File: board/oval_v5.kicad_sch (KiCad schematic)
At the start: 125 parts, among them J1 HDR-5x1, J10 HDR-4x1, J11 HDR-4x1, J12 HDR-4x1, J13 HDR-4x1, J14 HDR-4x1, J15 HDR-4x1, J16 HDR-4x1, J17 HDR-4x1, J18 Conn_Coaxial, J19 Conn_01x02, J2 HDR-4x1, J20 Conn_01x02, J21 Conn_02x02_Counter_Clockwise, J22 HDR-2x1, J23 HDR-2x1, J25 Conn_01x06, J3 HDR-4x1, J4 Conn_01x06, J5 Micro_SD_Card, J6 Conn_01x02, J7 HDR-4x1, J8 Conn_01x08, J9 HDR-4x1, P1 USB_C_Plug_USB2.0, Q1 Q_PMOS_GSD, Q2 MMBT3904, Q3 MMBT3904, SW1 SW_DIP_x02, SW2 SW_DIP_x02, U1 RV-8803, U10 SiP32431DR3, U11 SiP32431DR3, U12 SiP32431DR3, U13 SiP32431DR3, U14 SiP32431DR3, U15 PCF8574TS, U16 PCA9548APW, U17 SiP32431DR3, U2 ESP32-S3-WROOM-1, U3 TMP117xxDRV, U4 RFM95W-915S2, U7 MAX3485, U8 AP7361C-33E, U9 AP7361C-33E

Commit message: assignint pines
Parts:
- removed U15: PCF8574TS, Package_SO:SSOP-20_4.4x6.5mm_P0.65mm, symbol Interface_Expansion:PCF8574TS
- added C33: 100n, Capacitor_SMD:C_0603_1608Metric, symbol IoWLabs:C
- added C34: 10u, Capacitor_SMD:C_0805_2012Metric, symbol IoWLabs:C
- added R34, R35: 10k, Resistor_SMD:R_0603_1608Metric, symbol Device:R
- added R36, R37: 10K, Resistor_SMD:R_0603_1608Metric, symbol IoWLabs:RES
- added U18: PCA9555PW, Package_SO:TSSOP-24_4.4x7.8mm_P0.65mm, symbol Interface_Expansion:PCA9555PW
- R10, R11: value 2.2k -> 10k
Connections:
- net SPI_CS is gone; now on net SD_CS: U2.18 (GPIO10/TOUCH10/ADC1_CH9/FSPICS0/FSPIIO4/SUBSPICS0)
- net EN_FAN_1: now also U18.10 (IO0_6)
- net EN_FAN_2: now also U18.11 (IO0_7)
- net GND: now also C33.2, C34.2, U18.12 (VSS), U18.2 (A1), U18.21 (A0), U18.3 (A2)
- net GSM_PWRKEY: now also U2.6 (GPIO6/TOUCH6/ADC1_CH5)
- net GSM_RST: now also U2.5 (GPIO5/TOUCH5/ADC1_CH4)
- net PMS_Rx: now also U2.35 (MTMS/GPIO42)
- net PMS_SET: now also U18.13 (IO1_0)
- net PMS_Tx: now also U2.34 (MTDI/GPIO41/CLK_OUT1)
- net RS485_EN: now also U18.14 (IO1_1); no longer U2.25 (GPIO48/SPICLK_N/SUBSPICLK_N_DIFF)
- net SCL: now also R35.2, R36.1, U18.22 (SCL)
- net SDA: now also R34.2, R37.1, U18.23 (SDA)
- net V_DL_EN: now also U18.6 (IO0_2)
- net V_GSM_EN: now also U18.9 (IO0_5)
- net V_L: now also C33.1, C34.1, R36.2, R37.2, U18.24 (VDD)
- net V_RF_EN: now also U18.5 (IO0_1)
- net V_S1_EN: now also U18.7 (IO0_3)
- net V_S2: now also R34.1, R35.1
- net V_S2_EN: now also U18.8 (IO0_4)
- net onBoard_LED: now also U18.4 (IO0_0)
- net rfm_CS: now also U2.33 (MTDO/GPIO40/CLK_OUT2); no longer U2.4 (GPIO4/TOUCH4/ADC1_CH3)
- net rfm_RST: now also U2.32 (MTCK/GPIO39/CLK_OUT3/SUBSPICS1); no longer U2.5 (GPIO5/TOUCH5/ADC1_CH4)
- net rfm_dio0: now also U2.31 (GPIO38/FSPIWP/SUBSPIWP); no longer U2.23 (GPIO21)
- net rfm_dio2: now also U2.25 (GPIO48/SPICLK_N/SUBSPICLK_N_DIFF); no longer U2.6 (GPIO6/TOUCH6/ADC1_CH5)
- no-connect marks 23 -> 21
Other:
- note added: "Default I2C address : 0x20"
- note removed: "Default I2C address : 0x50"
- moved on the sheet: C5, C6, J4, J7, J9, R6, R8

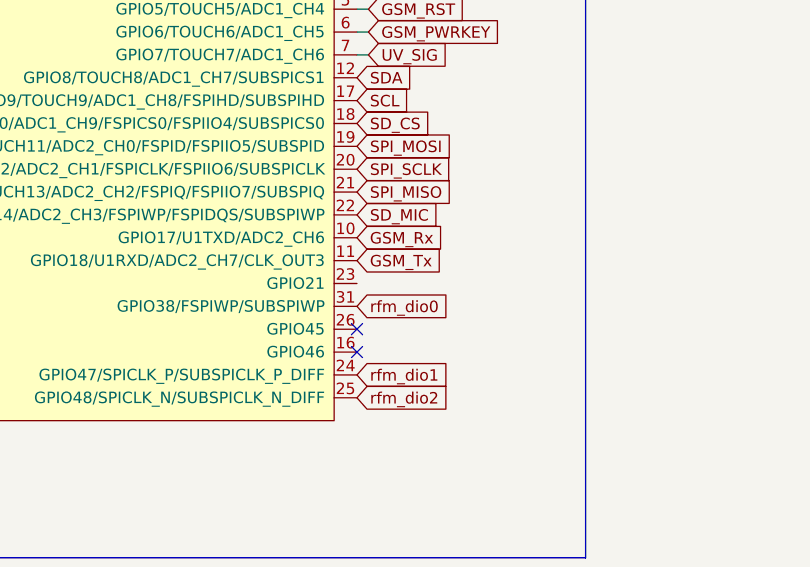
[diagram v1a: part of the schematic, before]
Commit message: updateing 27/02
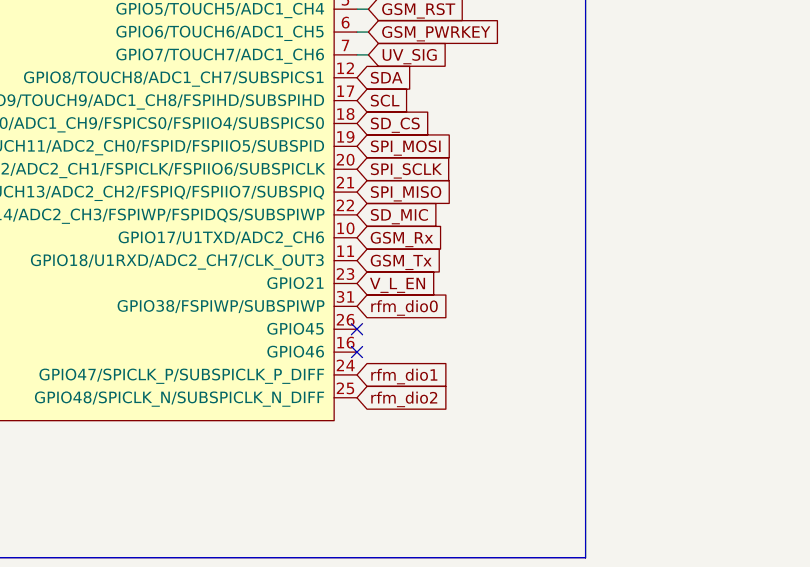
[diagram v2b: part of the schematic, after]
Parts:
- J1: footprint Connector_JST:JST_XH_B5B-XH-A_1x05_P2.50mm_Vertical -> Connector_JST:JST_PH_B5B-PH-K_1x05_P2.00mm_Vertical
- J10, J11, J12, J13, J14, J15, J16, J17: footprint Connector_JST:JST_SH_BM04B-SRSS-TB_1x04-1MP_P1.00mm_Vertical -> Connector_JST:JST_PH_B4B-PH-K_1x04_P2.00mm_Vertical
- J2, J3: footprint Connector_JST:JST_XH_B4B-XH-A_1x04_P2.50mm_Vertical -> Connector_JST:JST_SH_BM04B-SRSS-TB_1x04-1MP_P1.00mm_Vertical
- J20: footprint Connector_JST:JST_XH_B2B-XH-A_1x02_P2.50mm_Vertical -> Connector_JST:JST_PH_B2B-PH-K_1x02_P2.00mm_Vertical
- J22, J23: footprint Connector_JST:JST_XH_B2B-XH-A_1x02_P2.50mm_Vertical -> Connector_JST:JST_PH_S2B-PH-SM4-TB_1x02-1MP_P2.00mm_Horizontal
- J7, J9: footprint Connector_JST:JST_XH_B4B-XH-A_1x04_P2.50mm_Vertical -> Connector_JST:JST_PH_B4B-PH-K_1x04_P2.00mm_Vertical
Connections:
- net V_L_EN: now also U2.23 (GPIO21)
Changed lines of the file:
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@@
 		)
 	)
+	(global_label "V_L_EN"
+		(shape input)
+		(at 187.96 134.62 0)
+		(fields_autoplaced yes)
+		(effects
+			(font
+				(size 1.27 1.27)
+			)
+			(justify left)
+		)
+		(property "Intersheetrefs" "${INTERSHEET_REFS}"
+			(at 197.4766 134.62 0)
+			(effects
+				(font
+					(size 1.27 1.27)
+				)
+				(justify left)
+				(hide yes)
+			)
+		)
+	)
 	(global_label "V_RF"
 		(shape input)
@@
 			)
 		)
-		(property "Footprint" "Connector_JST:JST_SH_BM04B-SRSS-TB_1x04-1MP_P1.00mm_Vertical"
+		(property "Footprint" "Connector_JST:JST_PH_B4B-PH-K_1x04_P2.00mm_Vertical"
 			(at 207.01 200.66 0)
 			(effects
@@
 			)
 		)
-		(property "Footprint" "Connector_JST:JST_SH_BM04B-SRSS-TB_1x04-1MP_P1.00mm_Vertical"
+		(property "Footprint" "Connector_JST:JST_PH_B4B-PH-K_1x04_P2.00mm_Vertical"
 			(at 170.18 238.76 0)
 			(effects
@@
 			)
 		)
-		(property "Footprint" "Connector_JST:JST_SH_BM04B-SRSS-TB_1x04-1MP_P1.00mm_Vertical"
+		(property "Footprint" "Connector_JST:JST_PH_B4B-PH-K_1x04_P2.00mm_Vertical"
 			(at 207.01 256.54 0)
 			(effects
@@
 			)
 		)
-		(property "Footprint" "Connector_JST:JST_XH_B4B-XH-A_1x04_P2.50mm_Vertical"
+		(property "Footprint" "Connector_JST:JST_PH_B4B-PH-K_1x04_P2.00mm_Vertical"
 			(at 101.6 251.46 0)
 			(effects
@@
 			)
 		)
-		(property "Footprint" "Connector_JST:JST_XH_B4B-XH-A_1x04_P2.50mm_Vertical"
+		(property "Footprint" "Connector_JST:JST_PH_B4B-PH-K_1x04_P2.00mm_Vertical"
 			(at 128.27 251.46 0)
 			(effects
@@
 			)
 		)
-		(property "Footprint" "Connector_JST:JST_SH_BM04B-SRSS-TB_1x04-1MP_P1.00mm_Vertical"
+		(property "Footprint" "Connector_JST:JST_PH_B4B-PH-K_1x04_P2.00mm_Vertical"
 			(at 170.18 257.81 0)
 			(effects
@@
 			)
 		)
-		(property "Footprint" "Connector_JST:JST_SH_BM04B-SRSS-TB_1x04-1MP_P1.00mm_Vertical"
+		(property "Footprint" "Connector_JST:JST_PH_B4B-PH-K_1x04_P2.00mm_Vertical"
 			(at 170.18 199.39 0)
 			(effects
@@
 			)
 		)
-		(property "Footprint" "Connector_JST:JST_XH_B2B-XH-A_1x02_P2.50mm_Vertical"
+		(property "Footprint" "Connector_JST:JST_PH_S2B-PH-SM4-TB_1x02-1MP_P2.00mm_Horizontal"
 			(at 302.26 236.22 0)
 			(effects
@@
 			)
 		)
-		(property "Footprint" "Connector_JST:JST_SH_BM04B-SRSS-TB_1x04-1MP_P1.00mm_Vertical"
+		(property "Footprint" "Connector_JST:JST_PH_B4B-PH-K_1x04_P2.00mm_Vertical"
 			(at 207.01 220.98 0)
 			(effects
@@
 			)
 		)
-		(property "Footprint" "Connector_JST:JST_SH_BM04B-SRSS-TB_1x04-1MP_P1.00mm_Vertical"
+		(property "Footprint" "Connector_JST:JST_PH_B4B-PH-K_1x04_P2.00mm_Vertical"
 			(at 170.18 219.71 0)
 			(effects
@@
 			)
 		)
-		(property "Footprint" "Connector_JST:JST_XH_B4B-XH-A_1x04_P2.50mm_Vertical"
+		(property "Footprint" "Connector_JST:JST_SH_BM04B-SRSS-TB_1x04-1MP_P1.00mm_Vertical"
 			(at 46.99 219.71 0)
 			(effects
@@
 			)
 		)
-		(property "Footprint" "Connector_JST:JST_XH_B2B-XH-A_1x02_P2.50mm_Vertical"
+		(property "Footprint" "Connector_JST:JST_PH_S2B-PH-SM4-TB_1x02-1MP_P2.00mm_Horizontal"
 			(at 302.26 193.04 0)
 			(effects
@@
 			)
 		)
-		(property "Footprint" "Connector_JST:JST_SH_BM04B-SRSS-TB_1x04-1MP_P1.00mm_Vertical"
+		(property "Footprint" "Connector_JST:JST_PH_B4B-PH-K_1x04_P2.00mm_Vertical"
 			(at 207.01 240.03 0)
 			(effects
@@
 			)
 		)
-		(property "Footprint" "Connector_JST:JST_XH_B2B-XH-A_1x02_P2.50mm_Vertical"
+		(property "Footprint" "Connector_JST:JST_PH_B2B-PH-K_1x02_P2.00mm_Vertical"
 			(at 269.24 35.56 0)
 			(effects
@@
 			)
 		)
-		(property "Footprint" "Connector_JST:JST_XH_B5B-XH-A_1x05_P2.50mm_Vertical"
+		(property "Footprint" "Connector_JST:JST_PH_B5B-PH-K_1x05_P2.00mm_Vertical"
 			(at 44.45 209.55 0)
 			(effects
@@
 			)
 		)
-		(property "Footprint" "Connector_JST:JST_XH_B4B-XH-A_1x04_P2.50mm_Vertical"
+		(property "Footprint" "Connector_JST:JST_SH_BM04B-SRSS-TB_1x04-1MP_P1.00mm_Vertical"
 			(at 48.26 292.1 0)
 			(effects
